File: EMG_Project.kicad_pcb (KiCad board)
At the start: 4 copper layers, 97.1 x 32.3 mm, 77 parts, among them J1 Conn_01x03, J10 Conn_01x01, J11 Conn_01x01, J12 Conn_01x02, J14 Conn_01x01, J15 Conn_01x01, J17 Conn_01x03, J18 Conn_01x02, J2 Conn_01x06, J4 Conn_01x01, J5 Conn_01x01, J6 Conn_01x01, J7 Conn_01x01, J8 Conn_01x01, J9 SJ1-3523N, SW1 SW_SPST, U1 MP2322GQH-Z, U2 ATTINY13-20SSU, U3 AMPLIFIER-INA331DGK_MSOP8, U4 OPA333AIDBVR, U5 OPA333AIDBVR, U6 CJ432

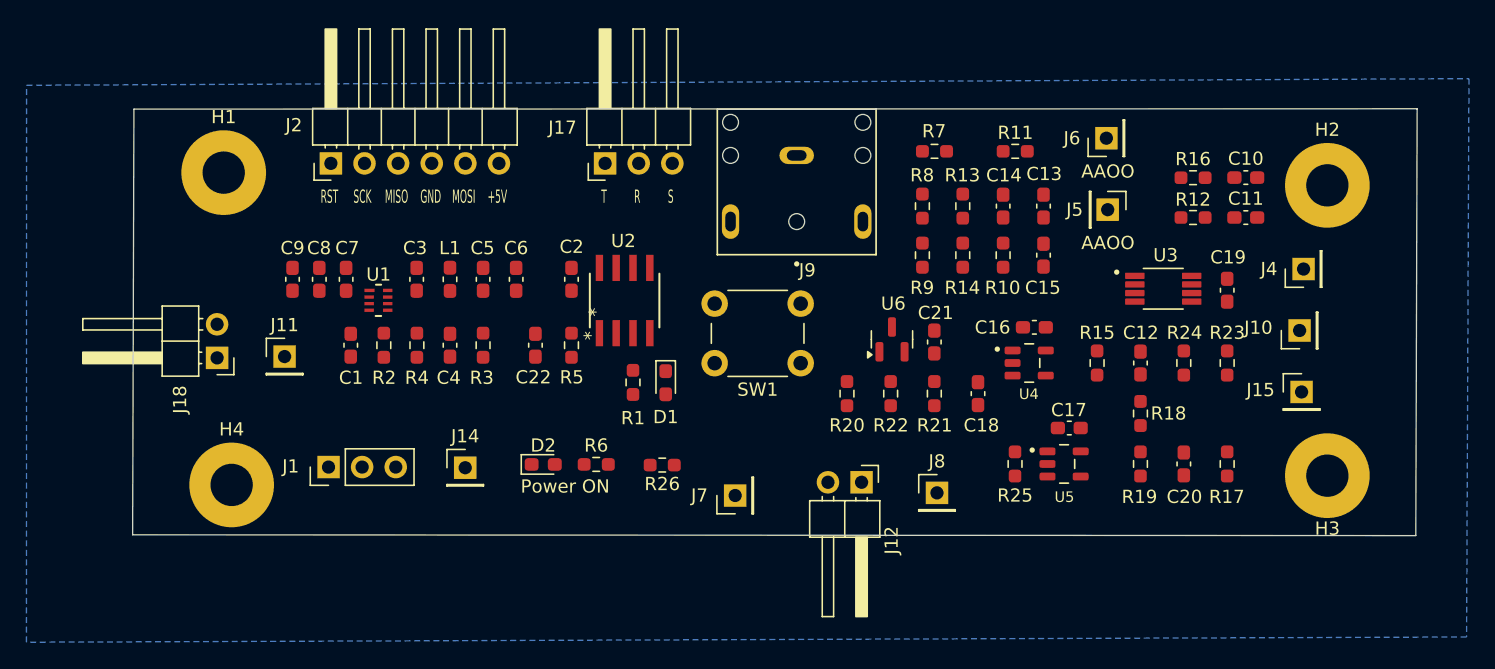
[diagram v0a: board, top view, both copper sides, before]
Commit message: Everything prepared for routing
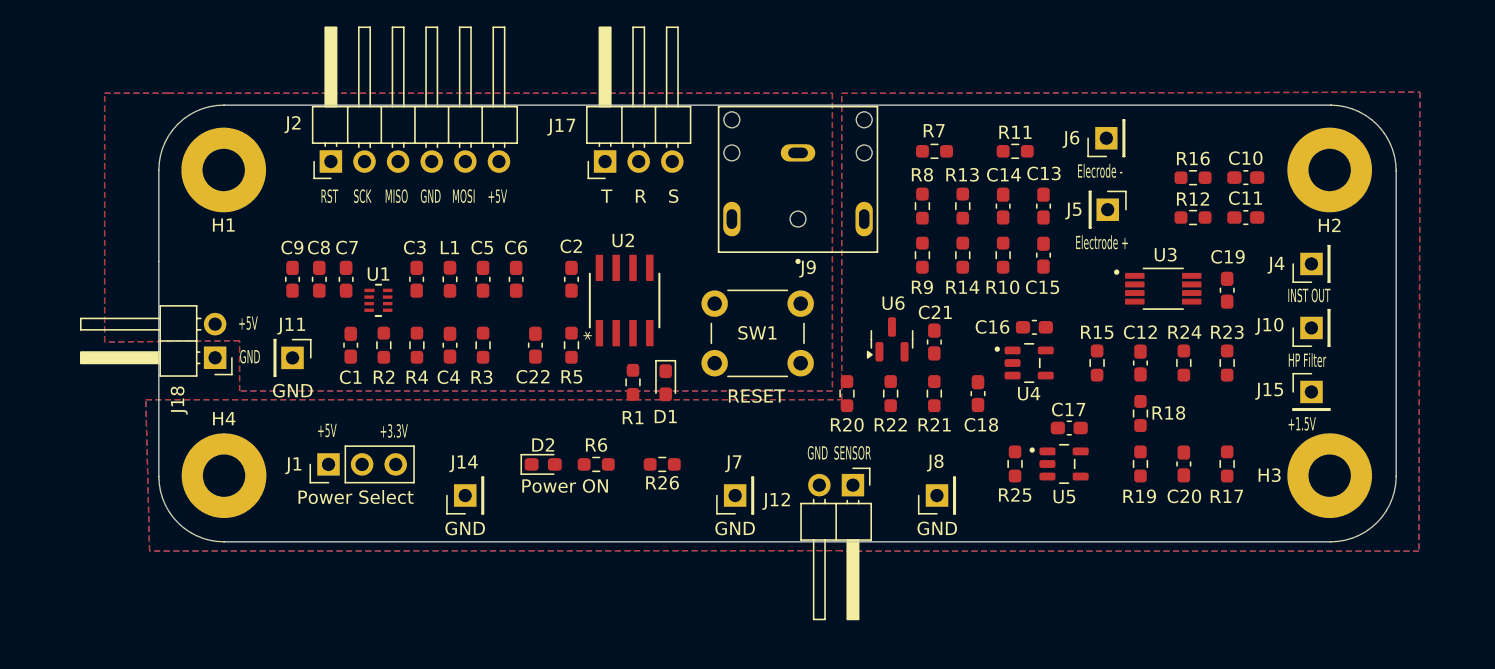
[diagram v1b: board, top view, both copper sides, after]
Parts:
- moved J14 2.10 mm to (85.7, 67.5), turned to 90 degrees
- moved H2 1.17 mm to (151.0, 42.9)
- moved J10 0.92 mm to (149.6, 54.8)
- moved H4 0.91 mm to (67.4, 66.0)
- moved J15 0.75 mm to (149.6, 59.7)
- moved J4 0.71 mm to (149.6, 50.0)
- moved J12 0.68 mm to (115.0, 66.7)
- moved J11 0.61 mm to (72.6, 57.1), turned to -90 degrees
- moved J9 0.21 mm to (110.8, 41.6)
- moved H1 0.20 mm to (67.4, 42.9)
- moved J8 0.20 mm to (121.3, 67.5), turned to 90 degrees
- moved J1 0.20 mm to (75.3, 65.2)
- moved H3 0.17 mm to (151.0, 66.0)
- moved J18 0.15 mm to (66.8, 57.1)
- moved J17 0.13 mm to (96.2, 42.3)
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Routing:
- net GND: track 0.00 -> 6.31 mm
- added copper zone on F.Cu, net GND
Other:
- board size 97.1 x 32.3 mm -> 93.5 x 33 mm
- board text added: "+1.5V"
- board text added: "+3.3V"
- board text added: "EMG Project version 1.0 30.04.2025"
- board text added: "Elecrode -"
- board text added: "Electrode +"
- board text added: "HP Filter"
- board text added: "INST OUT"
- board text added: "Power Select"
- board text added: "RESET"
- board text added: "SENSOR"
- board text removed: "AAOO"
